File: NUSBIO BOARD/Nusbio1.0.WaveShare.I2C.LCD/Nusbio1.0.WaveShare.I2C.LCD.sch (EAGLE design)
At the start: 14 parts

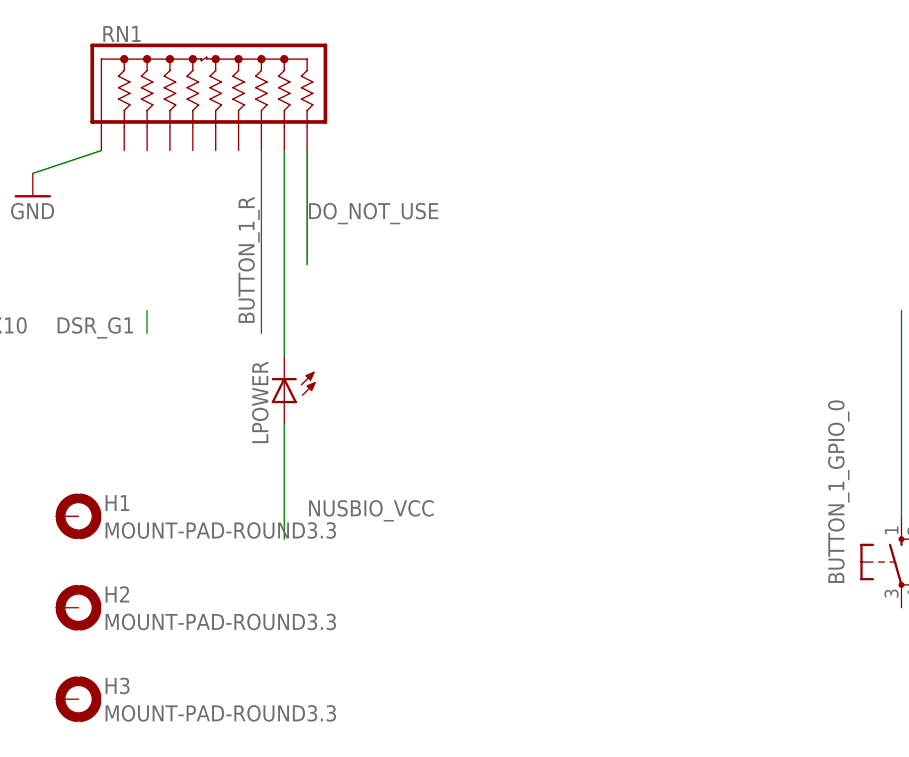
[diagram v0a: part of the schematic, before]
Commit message: Update...
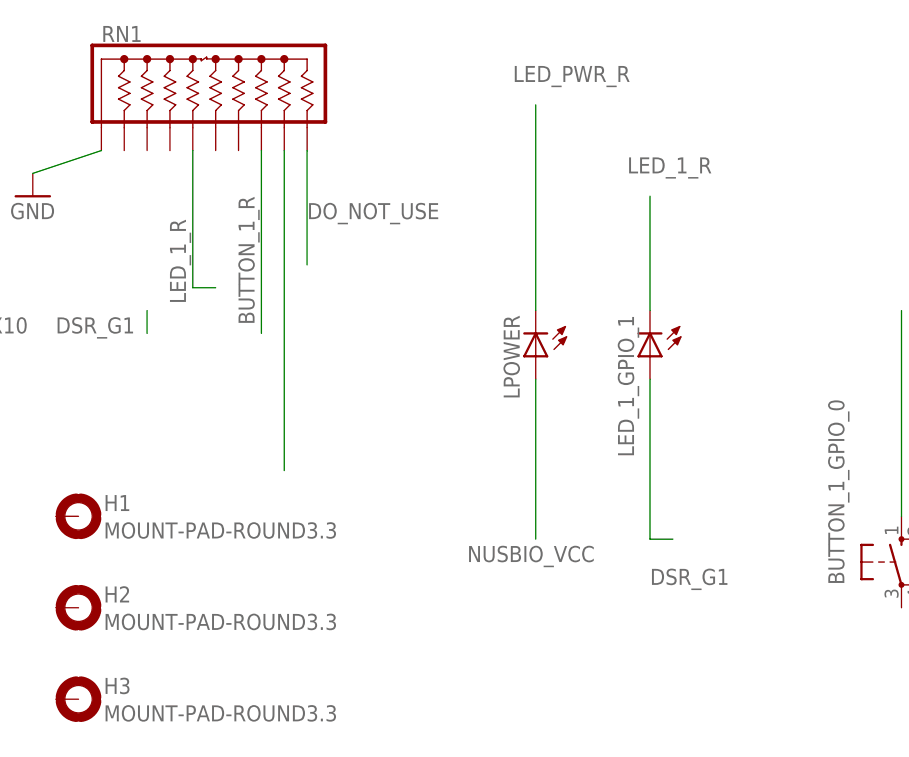
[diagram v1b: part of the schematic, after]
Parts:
- added LED_1_GPIO_1: (no value), adafruit:LEDSMT1206
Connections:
- net N$1 renamed LED_PWR_R
- new net LED_1_R: LED_1_GPIO_1.C, RN1.5
- net DSR_G1: now also LED_1_GPIO_1.A
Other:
- moved on the sheet: LPOWER
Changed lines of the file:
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@@
 <part name="H6" library="holes" library_urn="urn:adsk.eagle:library:237" deviceset="MOUNT-PAD-ROUND" device="3.3" package3d_urn="urn:adsk.eagle:package:14283/1"/>
 <part name="BUTTON_1_GPIO_0" library="switch-omron" library_urn="urn:adsk.eagle:library:377" deviceset="10-XX" device="" package3d_urn="urn:adsk.eagle:package:27496/1"/>
+<part name="LED_1_GPIO_1" library="adafruit" deviceset="LED" device="SMT1206"/>
 </parts>
 <sheets>
@@
 <attribute name="VALUE" x="142.24" y="68.58" size="1.778" layer="96"/>
 </instance>
-<instance part="LPOWER" gate="G$1" x="172.72" y="48.26" smashed="yes" rot="R180">
-<attribute name="NAME" x="169.164" y="52.832" size="1.778" layer="95" rot="R270"/>
-<attribute name="VALUE" x="167.005" y="52.832" size="1.778" layer="96" rot="R270"/>
+<instance part="LPOWER" gate="G$1" x="200.66" y="53.34" smashed="yes" rot="R180">
+<attribute name="NAME" x="197.104" y="57.912" size="1.778" layer="95" rot="R270"/>
+<attribute name="VALUE" x="194.945" y="57.912" size="1.778" layer="96" rot="R270"/>
 </instance>
 <instance part="H1" gate="G$1" x="149.86" y="35.56" smashed="yes">
@@
 <attribute name="NAME" x="234.95" y="27.94" size="1.778" layer="95" rot="R90"/>
 <attribute name="VALUE" x="237.49" y="33.655" size="1.778" layer="96" rot="R90"/>
+</instance>
+<instance part="LED_1_GPIO_1" gate="G$1" x="213.36" y="53.34" smashed="yes" rot="R180">
+<attribute name="NAME" x="209.804" y="57.912" size="1.778" layer="95" rot="R270"/>
+<attribute name="VALUE" x="207.645" y="57.912" size="1.778" layer="96" rot="R270"/>
 </instance>
 </instances>
@@
 <segment>
 <pinref part="LPOWER" gate="G$1" pin="A"/>
-<wire x1="172.72" y1="45.72" x2="172.72" y2="33.02" width="0.1524" layer="91"/>
-<label x="175.26" y="35.56" size="1.778" layer="95"/>
+<wire x1="200.66" y1="50.8" x2="200.66" y2="33.02" width="0.1524" layer="91"/>
+<label x="193.04" y="30.48" size="1.778" layer="95"/>
 </segment>
 <segment>
@@
 <label x="147.32" y="55.88" size="1.778" layer="95"/>
 </segment>
+<segment>
+<pinref part="LED_1_GPIO_1" gate="G$1" pin="A"/>
+<wire x1="213.36" y1="50.8" x2="213.36" y2="33.02" width="0.1524" layer="91"/>
+<wire x1="213.36" y1="33.02" x2="215.9" y2="33.02" width="0.1524" layer="91"/>
+<label x="213.36" y="27.94" size="1.778" layer="95"/>
+</segment>
 </net>
 <net name="RI_G0" class="0">
@@
 </segment>
 </net>
-<net name="N$1" class="0">
-<segment>
-<pinref part="LPOWER" gate="G$1" pin="C"/>
-<pinref part="RN1" gate="G$1" pin="9"/>
-<wire x1="172.72" y1="53.34" x2="172.72" y2="76.2" width="0.1524" layer="91"/>
-</segment>
-</net>
 <net name="BUTTON_1_R" class="0">
 <segment>
@@
 </segment>
 </net>
+<net name="LED_1_R" class="0">
+<segment>
+<pinref part="RN1" gate="G$1" pin="5"/>
+<wire x1="162.56" y1="76.2" x2="162.56" y2="60.96" width="0.1524" layer="91"/>
+<wire x1="162.56" y1="60.96" x2="165.1" y2="60.96" width="0.1524" layer="91"/>
+<label x="160.02" y="68.58" size="1.778" layer="95" rot="R270"/>
+</segment>
+<segment>
+<pinref part="LED_1_GPIO_1" gate="G$1" pin="C"/>
+<wire x1="213.36" y1="58.42" x2="213.36" y2="71.12" width="0.1524" layer="91"/>
+<label x="210.82" y="73.66" size="1.778" layer="95"/>
+</segment>
+</net>
+<net name="LED_PWR_R" class="0">
+<segment>
+<pinref part="RN1" gate="G$1" pin="9"/>
+<wire x1="172.72" y1="76.2" x2="172.72" y2="40.64" width="0.1524" layer="91"/>
+</segment>
+<segment>
+<pinref part="LPOWER" gate="G$1" pin="C"/>
+<wire x1="200.66" y1="58.42" x2="200.66" y2="81.28" width="0.1524" layer="91"/>
+<label x="198.12" y="83.82" size="1.778" layer="95"/>
+</segment>
+</net>
